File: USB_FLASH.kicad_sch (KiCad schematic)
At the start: 26 parts, among them J5 USB_C_UART, J6 USB_C_OTG, Q1 BC847, Q2 BC847, U10 USBLC6-2SC6, U11 CP2102N, U12 USBLC6-2SC6

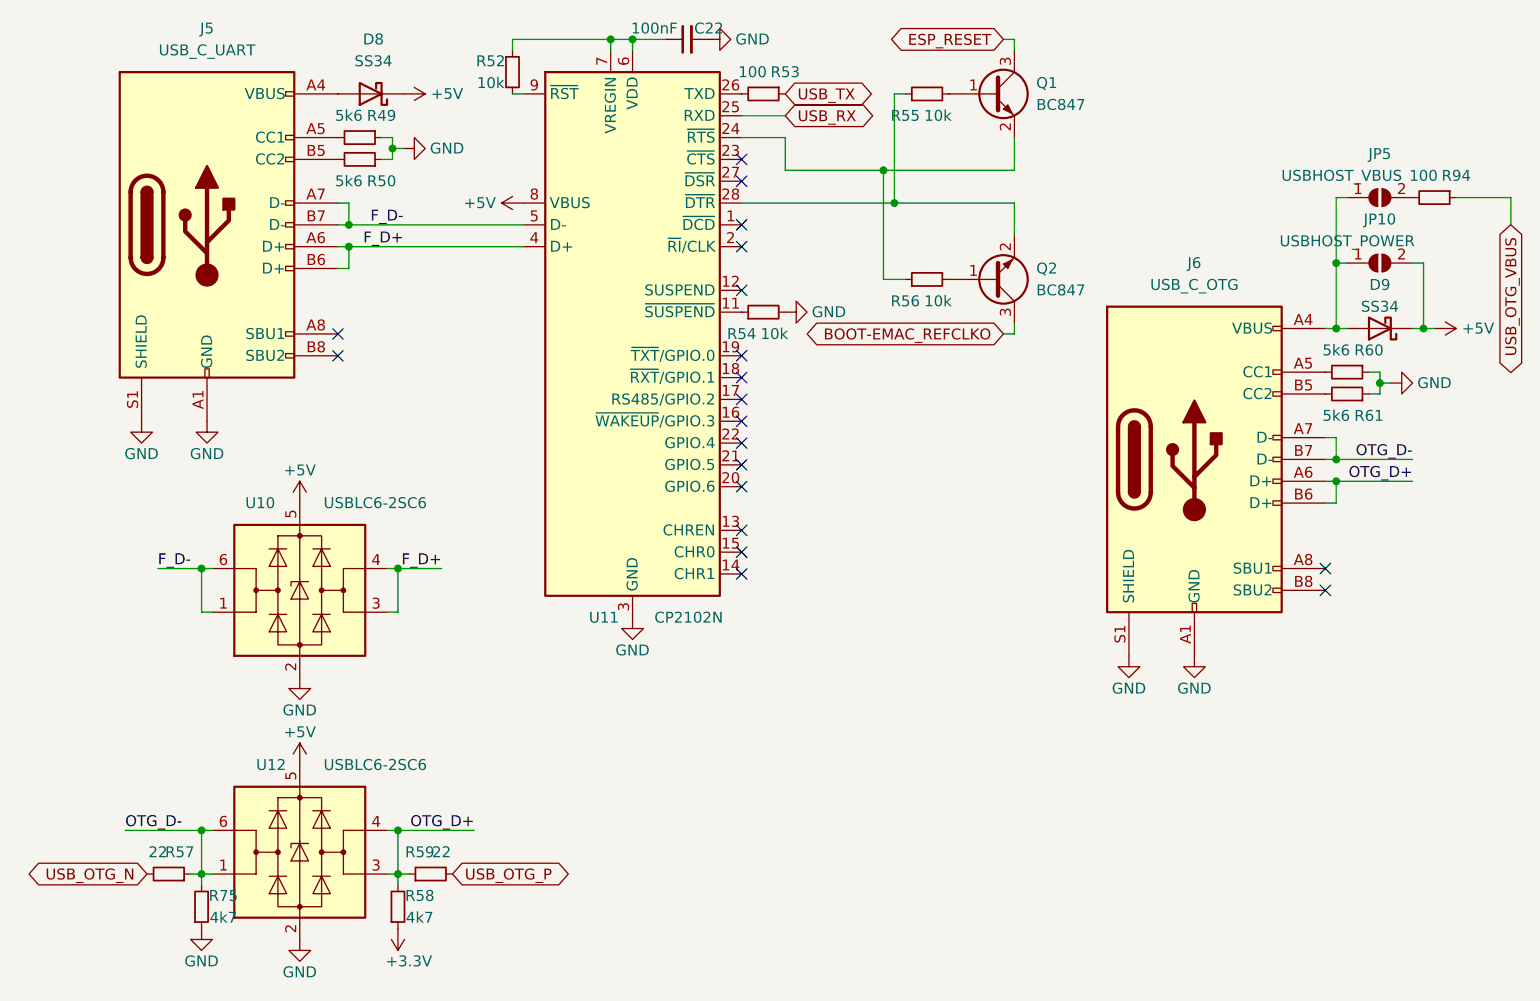
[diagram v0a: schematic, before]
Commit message: Add files via upload
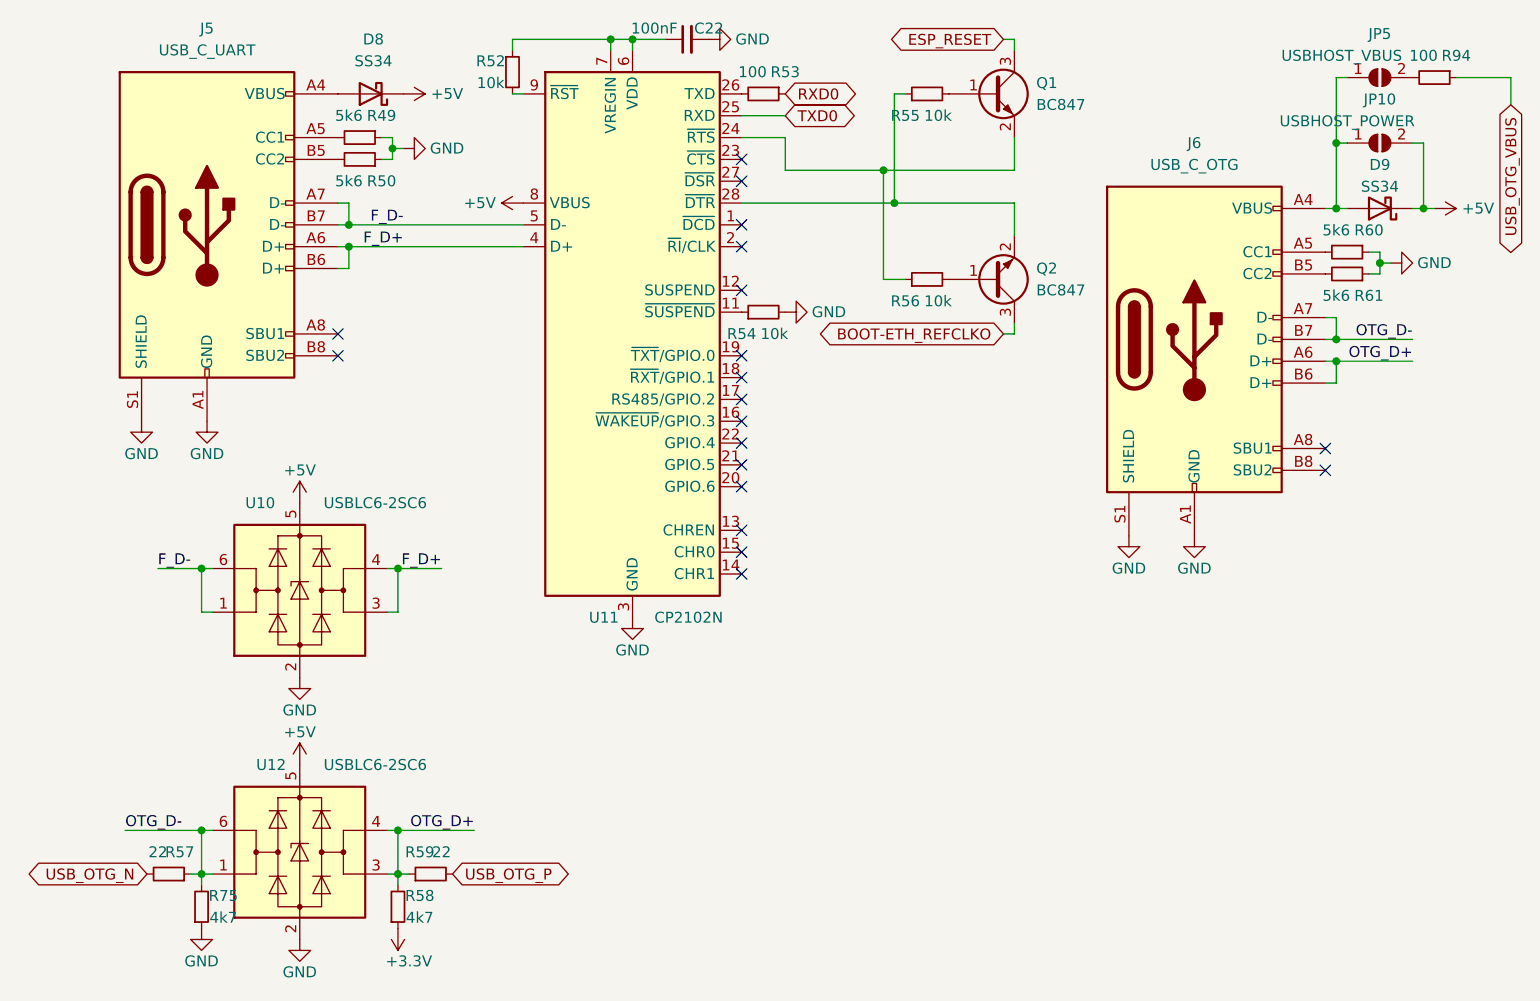
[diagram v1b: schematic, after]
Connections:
- net BOOT-EMAC_REFCLKO renamed BOOT-ETH_REFCLKO
- net USB_RX renamed TXD0
- net USB_TX renamed RXD0
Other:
- moved on the sheet: D9, J6, JP10, JP5, R60, R61, R94
